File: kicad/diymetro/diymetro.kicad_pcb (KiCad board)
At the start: 2 copper layers, 162.8 x 100 mm, 113 parts, among them J1 AudioJack2_SwitchT, J2 AudioJack2_SwitchT, J3 AudioJack2_SwitchT, J4 AudioJack2_SwitchT, J5 Conn_02x08_Top_Bottom, J6 AudioJack2_SwitchT, J7 ICSP, J8 SER, Q1 MMBT2222A, Q2 MMBT2222A, SW1 SW_SPDT_MSM, SW10 SW_Push, SW2 SW_SPDT_MSM, SW3 SW_SPDT_MSM, SW4 SW_SPDT_MSM, SW5 SW_SPDT_MSM, SW6 SW_SPDT_MSM, SW7 SW_SPDT_MSM, SW8 SW_SPDT_MSM, SW9 SW_Rotary12, U1 74HC4051, U2 74LS595, U3 74HC4051, U4 74HC4051, U5 ATmega328P-PU, Y1 Crystal

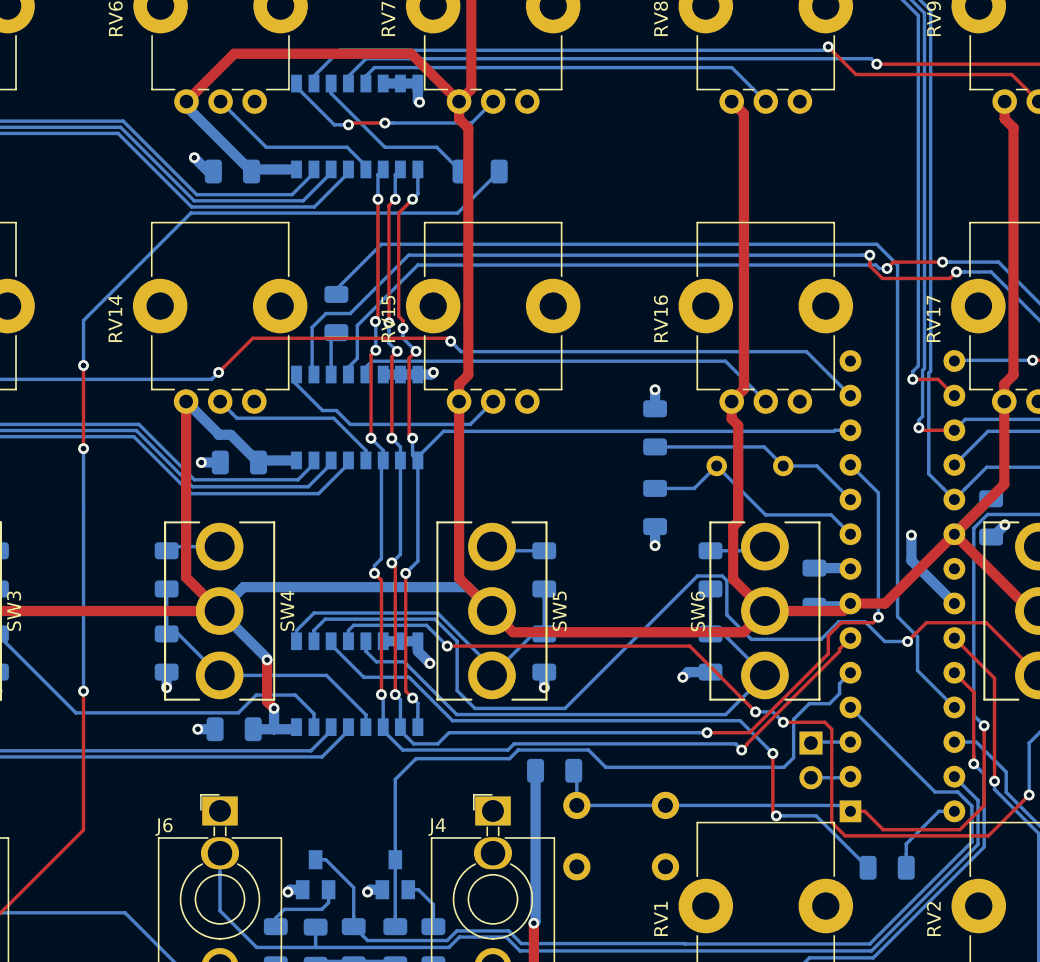
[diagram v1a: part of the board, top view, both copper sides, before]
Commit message: Remove some unused diodes.
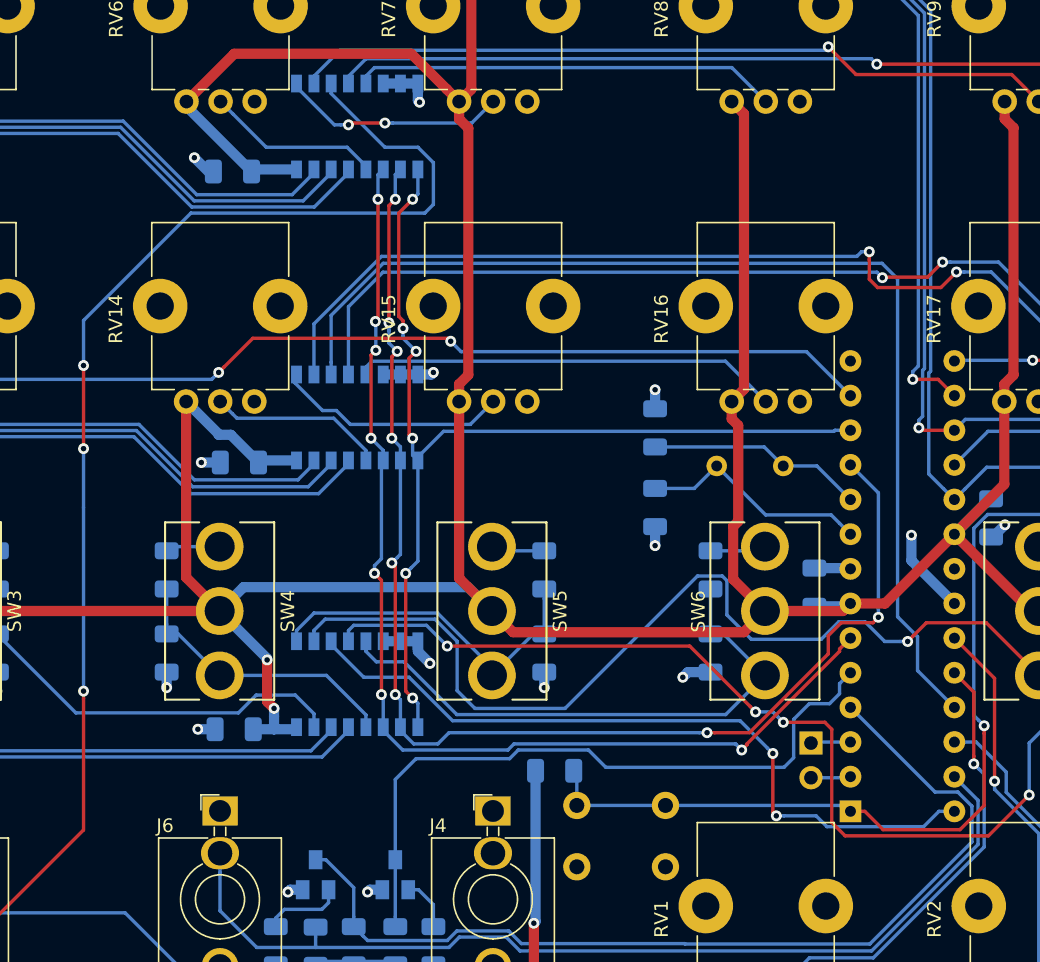
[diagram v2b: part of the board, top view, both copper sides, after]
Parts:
- removed D12, D13, D3: D, Diode_SMD:D_1206_3216Metric
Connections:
- U1 pad 3: Net-(D3-Pad2) -> SA
- U3 pad 3: Net-(D12-Pad2) -> PIN_CVOUT
- U4 pad 3: Net-(D13-Pad2) -> PIN_GATEOUT
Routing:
- net Net-(D3-Pad2): track 48.9 -> 0.00 mm, vias 2 -> 0
- net SA: track 6.26 -> 54.5 mm, vias 0 -> 2
- net Net-(D12-Pad2): track 12.6 -> 0.00 mm
- net PIN_CVOUT: track 86.5 -> 94.1 mm
- net PIN_GATEOUT: track 77.7 -> 81.1 mm
- net Net-(D13-Pad2): track 3.23 -> 0.00 mm
- net /Gate Pots/GA6: track 68.5 -> 70.0 mm
- net /Gate Pots/GA7: track 81.6 -> 82.9 mm
